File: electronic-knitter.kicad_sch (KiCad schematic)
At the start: 36 parts, among them J101 SOLENOIDS, J103 USB_C_Receptacle_USB2.0, J104 STLINK B2B, J105 Conn_ST_STDC14, Q101 AO3400A, SW101 BOOT, SW102 RESET, U101 STM32F103C8Tx, U102 SRV05-4, Y101 12MHz

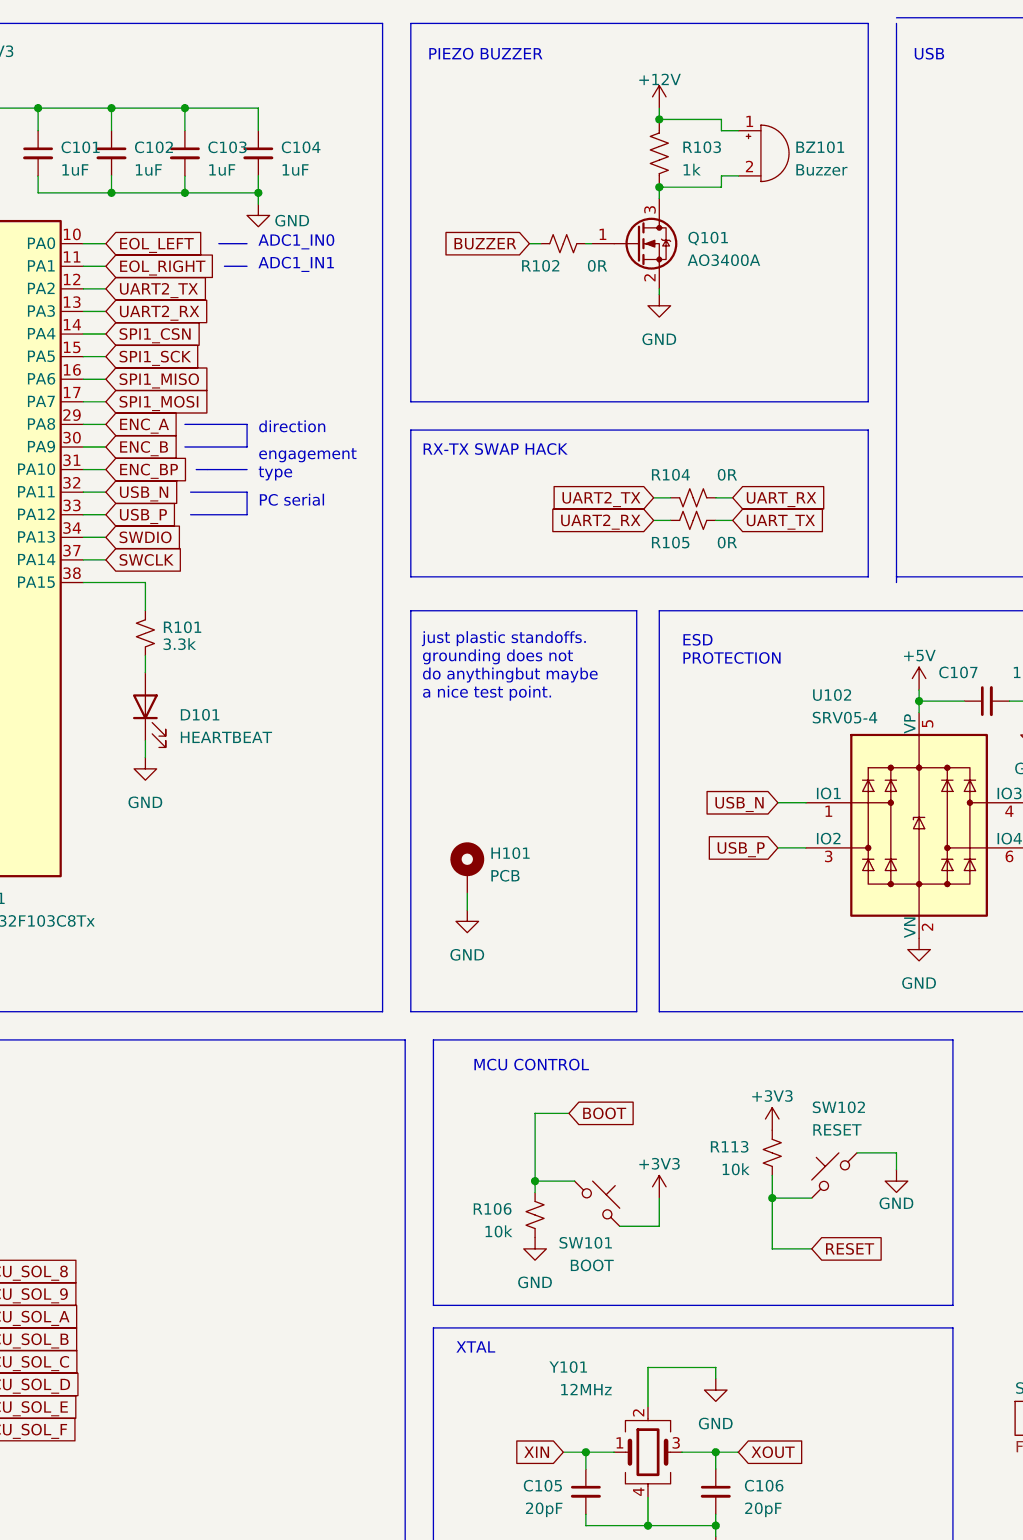
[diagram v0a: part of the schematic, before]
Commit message: finalize fab files and order first rev of board
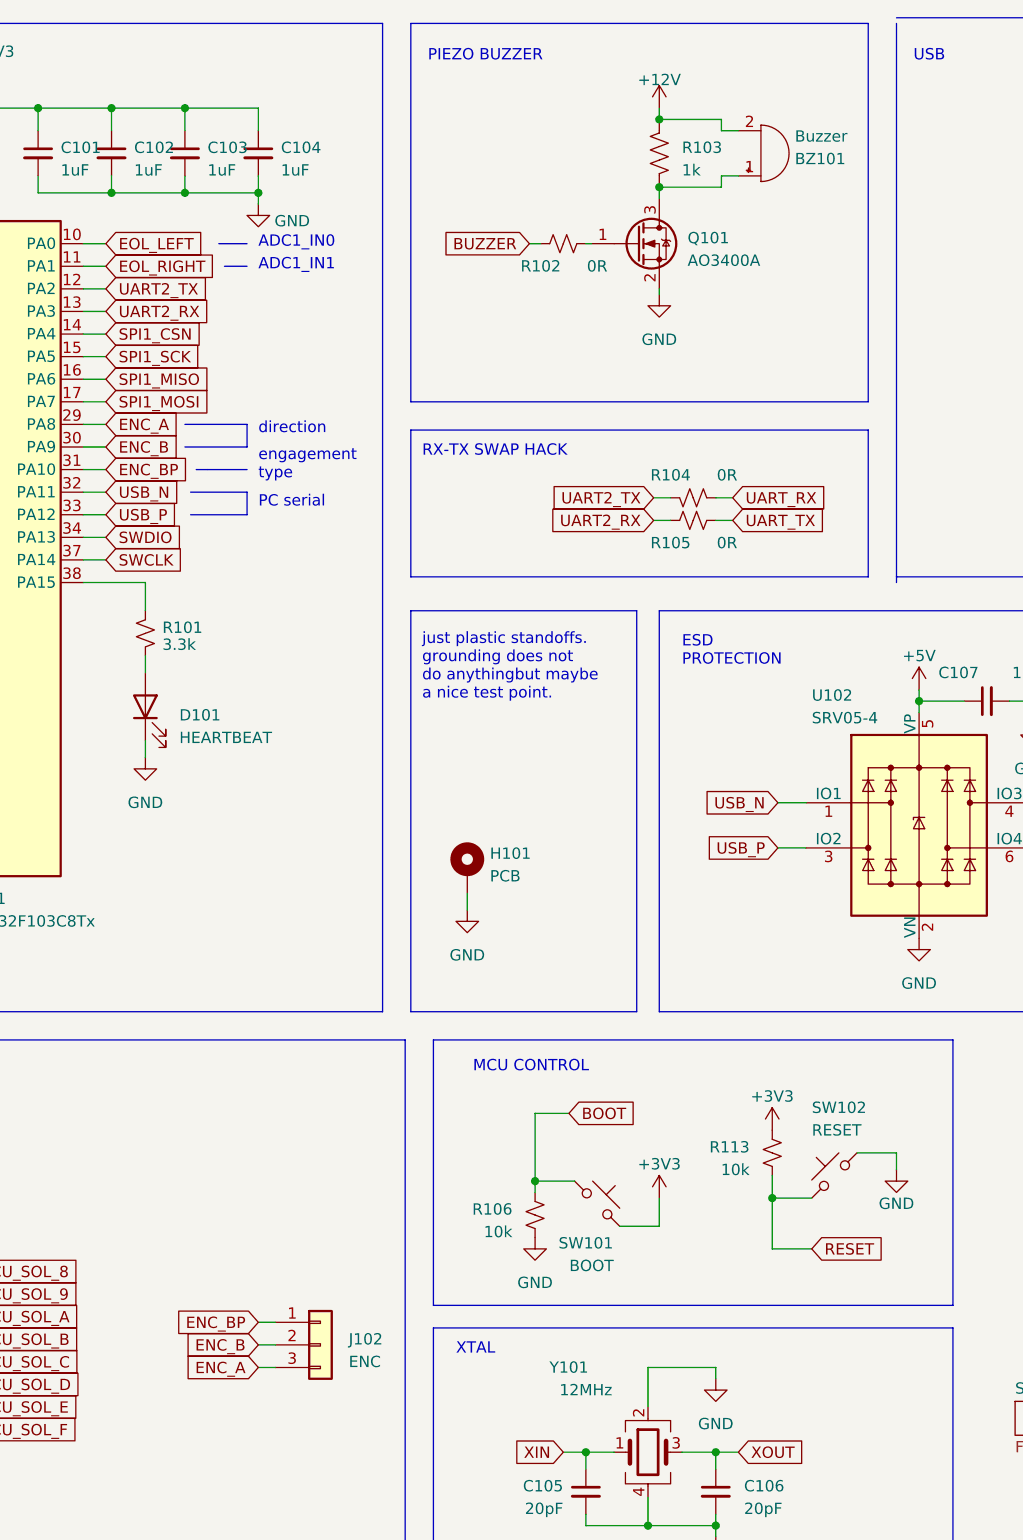
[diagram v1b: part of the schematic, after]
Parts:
- added J102: ENC, Connector_PinHeader_2.54mm:PinHeader_1x03_P2.54mm_Vertical, symbol Connector_Generic:Conn_01x03
- BZ101: footprint Buzzer_Beeper:Buzzer_12x9.5RM7.6 -> easyeda2kicad:BUZ-SMD_MLT-9032
- H101, J101: now left out of the parts list
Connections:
- net +12V: now also BZ101.2 (+); no longer BZ101.1 (-)
- net ENC_A: now also J102.3 (Pin_3)
- net ENC_B: now also J102.2 (Pin_2)
- net ENC_BP: now also J102.1 (Pin_1)
- net at Q101.3 (D), R103.2: now also BZ101.1 (-); no longer BZ101.2 (+)
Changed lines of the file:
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@@
+    (stroke (width 0) (type default))
+  )
+  (wire (pts (xy 95.25 161.925) (xy 97.155 161.925))
     (stroke (width 0) (type default))
   )
@@
     (stroke (width 0) (type default))
   )
+  (wire (pts (xy 95.25 167.005) (xy 97.155 167.005))
+    (stroke (width 0) (type default))
+  )
   (wire (pts (xy 146.685 167.005) (xy 146.685 168.275))
     (stroke (width 0) (type default))
@@
   )
   (polyline (pts (xy 112.395 15.875) (xy 112.395 58.42))
+    (stroke (width 0) (type default))
+  )
+  (wire (pts (xy 95.25 164.465) (xy 97.155 164.465))
     (stroke (width 0) (type default))
   )
@@
     )
   )
+  (global_label "ENC_B" (shape input) (at 95.25 164.465 180) (fields_autoplaced)
+    (effects (font (size 1.27 1.27)) (justify right))
+    (property "Intersheetrefs" "${INTERSHEET_REFS}" (at 86.3571 164.465 0)
+      (effects (font (size 1.27 1.27)) (justify right) hide)
+    )
+  )
   (global_label "ENC_BP" (shape input) (at 78.105 66.04 0) (fields_autoplaced)
     (effects (font (size 1.27 1.27)) (justify left))
@@
     )
   )
+  (global_label "ENC_BP" (shape input) (at 95.25 161.925 180) (fields_autoplaced)
+    (effects (font (size 1.27 1.27)) (justify right))
+    (property "Intersheetrefs" "${INTERSHEET_REFS}" (at 85.0871 161.925 0)
+      (effects (font (size 1.27 1.27)) (justify right) hide)
+    )
+  )
   (global_label "USB_P" (shape input) (at 153.67 108.585 180) (fields_autoplaced)
     (effects (font (size 1.27 1.27)) (justify right))
@@
     (property "Intersheetrefs" "${INTERSHEET_REFS}" (at 75.7796 173.99 0)
       (effects (font (size 1.27 1.27)) (justify left) hide)
+    )
+  )
+  (global_label "ENC_A" (shape input) (at 95.25 167.005 180) (fields_autoplaced)
+    (effects (font (size 1.27 1.27)) (justify right))
+    (property "Intersheetrefs" "${INTERSHEET_REFS}" (at 86.5385 167.005 0)
+      (effects (font (size 1.27 1.27)) (justify right) hide)
     )
   )
@@
         (path "/a3f4eded-ecb9-44ce-82ad-ad815e00f2c9"
           (reference "SW102") (unit 1)
+        )
+      )
+    )
+  )
+  (symbol (lib_id "Connector_Generic:Conn_01x03") (at 102.235 164.465 0) (unit 1)
+    (in_bom no) (on_board yes) (dnp no) (fields_autoplaced)
+    (property "Reference" "J102" (at 105.41 163.83 0)
+      (effects (font (size 1.27 1.27)) (justify left))
+    )
+    (property "Value" "ENC" (at 105.41 166.37 0)
+      (effects (font (size 1.27 1.27)) (justify left))
+    )
+    (property "Footprint" "Connector_PinHeader_2.54mm:PinHeader_1x03_P2.54mm_Vertical" (at 102.235 164.465 0)
+      (effects (font (size 1.27 1.27)) hide)
+    )
+    (property "Datasheet" "~" (at 102.235 164.465 0)
+      (effects (font (size 1.27 1.27)) hide)
+    )
+    (pin "1")
+    (pin "2")
+    (pin "3")
+    (instances
+      (project "electronic-knitter"
+        (path "/a3f4eded-ecb9-44ce-82ad-ad815e00f2c9"
+          (reference "J102") (unit 1)
         )
       )
@@
   )
   (symbol (lib_id "matei:HP_1650-63203_logicanalyzer") (at 48.26 161.29 0) (unit 1)
-    (in_bom yes) (on_board yes) (dnp no)
+    (in_bom no) (on_board yes) (dnp no)
     (property "Reference" "J101" (at 48.26 139.7 0)
       (effects (font (size 1.27 1.27)))
@@
   )
   (symbol (lib_id "Mechanical:MountingHole_Pad") (at 118.745 111.125 0) (unit 1)
-    (in_bom yes) (on_board yes) (dnp no) (fields_autoplaced)
+    (in_bom no) (on_board yes) (dnp no) (fields_autoplaced)
     (property "Reference" "H101" (at 121.285 109.22 0)
       (effects (font (size 1.27 1.27)) (justify left))
@@
     )
   )
-  (symbol (lib_id "Device:Buzzer") (at 151.765 30.48 0) (unit 1)
+  (symbol (lib_id "Device:Buzzer") (at 151.765 30.48 0) (mirror x) (unit 1)
     (in_bom yes) (on_board yes) (dnp no)
-    (property "Reference" "BZ101" (at 155.575 29.845 0)
-      (effects (font (size 1.27 1.27)) (justify left))
-    )
-    (property "Value" "Buzzer" (at 155.575 32.385 0)
-      (effects (font (size 1.27 1.27)) (justify left))
-    )
-    (property "Footprint" "Buzzer_Beeper:Buzzer_12x9.5RM7.6" (at 151.13 27.94 90)
-      (effects (font (size 1.27 1.27)) hide)
-    )
-    (property "Datasheet" "~" (at 151.13 27.94 90)
-      (effects (font (size 1.27 1.27)) hide)
-    )
+    (property "Reference" "BZ101" (at 155.575 31.115 0)
+      (effects (font (size 1.27 1.27)) (justify left))
+    )
+    (property "Value" "Buzzer" (at 155.575 28.575 0)
+      (effects (font (size 1.27 1.27)) (justify left))
+    )
+    (property "Footprint" "easyeda2kicad:BUZ-SMD_MLT-9032" (at 151.13 33.02 90)
+      (effects (font (size 1.27 1.27)) hide)
+    )
+    (property "Datasheet" "~" (at 151.13 33.02 90)
+      (effects (font (size 1.27 1.27)) hide)
+    )
